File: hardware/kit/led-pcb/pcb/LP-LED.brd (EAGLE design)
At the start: 15 x 15 mm, 2 parts

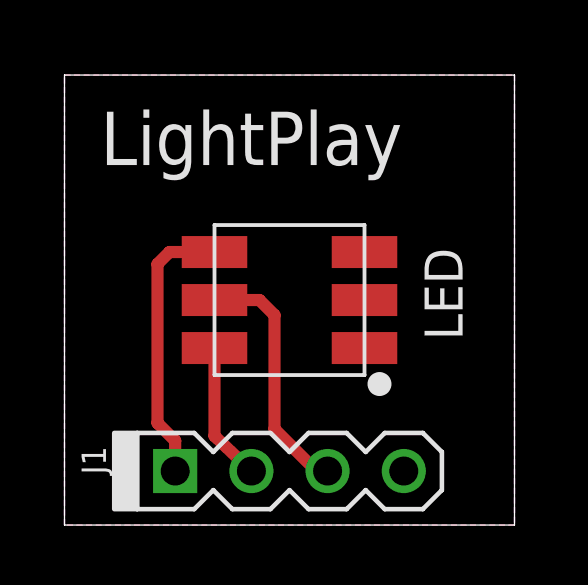
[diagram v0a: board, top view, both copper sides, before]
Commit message: rev-b pcb
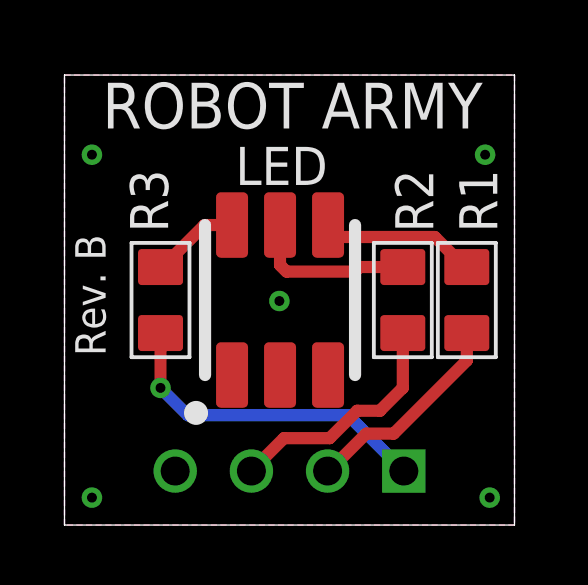
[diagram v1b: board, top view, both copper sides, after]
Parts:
- added R1, R3: 133, rlc:0805
- added R2: 200, rlc:0805
- moved LED 0.31 mm to (7.19, 7.50), turned to 90 degrees
- flipped J1 to the bottom
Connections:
- net GND renamed COMMON
- new net N$4: LED.5, R2.2
- new net N$5: J1.2, R1.1
- new net N$6: J1.1, R3.1
- net N$1: now also LED.4, R1.2; no longer J1.3, LED.5
- net N$2: now also J1.3, R2.1; no longer J1.2, LED.6
- net N$3: now also LED.6, R3.2; no longer J1.1, LED.4
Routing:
- net N$6: track 0.00 -> 11.1 mm, vias 0 -> 1
- net N$5: track 0.00 -> 7.08 mm
- net N$3: track 9.21 -> 2.96 mm
- net N$4: track 0.00 -> 5.58 mm
- net N$2: track 4.63 -> 8.03 mm
- net N$1: track 8.36 -> 5.50 mm
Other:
- board text added: "ROBOT ARMY"
- board text added: "Rev. B"
- board text removed: "=F"
- board text removed: "LightPlay"
